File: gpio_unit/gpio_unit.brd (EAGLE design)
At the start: 89.2 x 39.4 mm, 18 parts, among them X1 RASPI_GPIO_B+_PIN

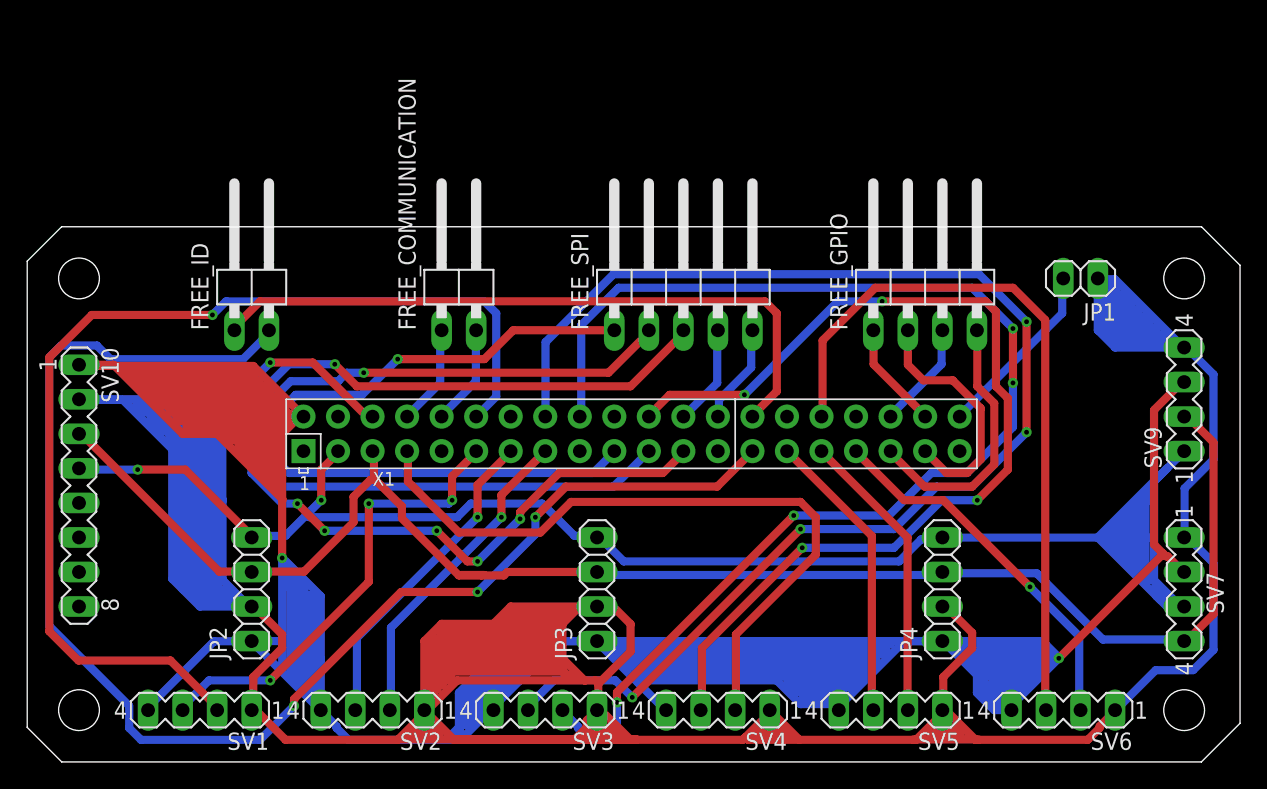
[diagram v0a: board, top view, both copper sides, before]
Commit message: arrange comment
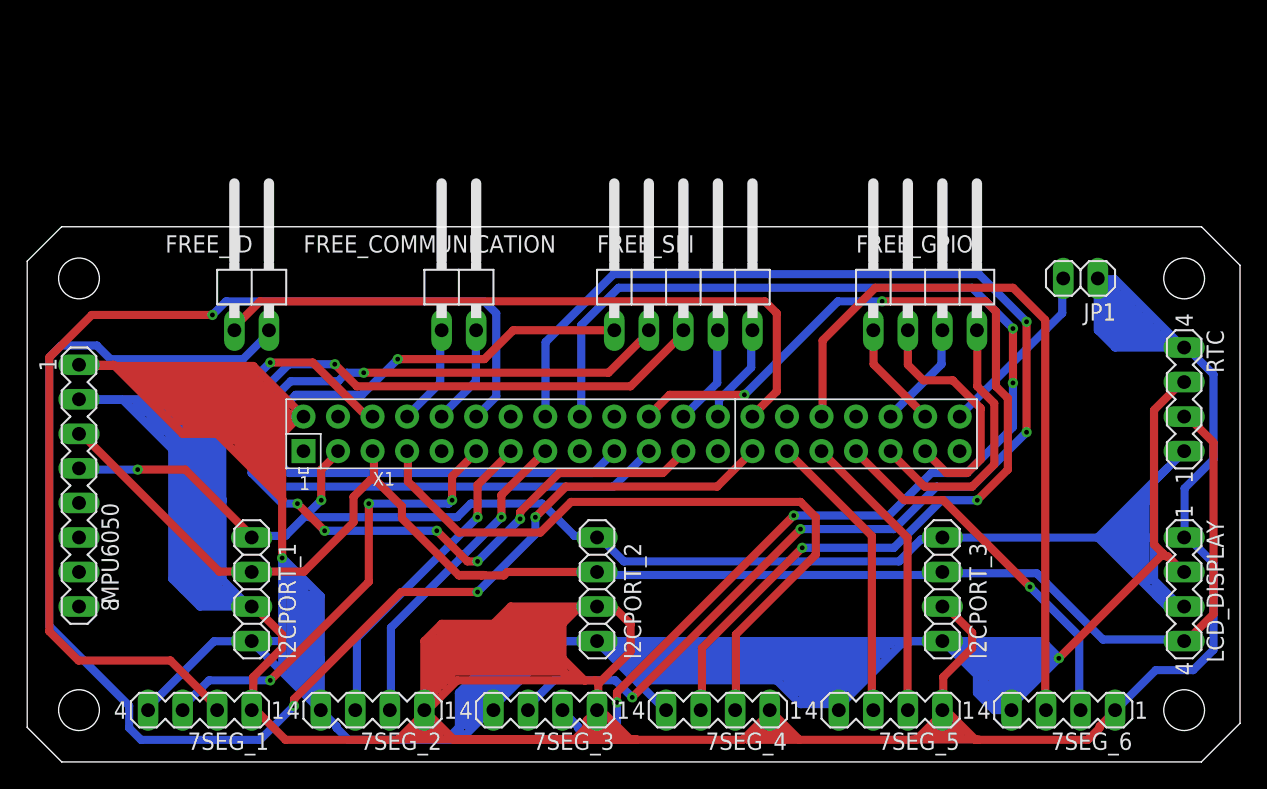
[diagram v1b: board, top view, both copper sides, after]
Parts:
- renumbered JP2 to I2CPORT_1, JP3 to I2CPORT_2, JP4 to I2CPORT_3, SV1 to 7SEG_1, SV10 to MPU6050, SV2 to 7SEG_2, SV3 to 7SEG_3, SV4 to 7SEG_4, SV5 to 7SEG_5, SV6 to 7SEG_6, SV7 to LCD_DISPLAY, SV9 to RTC
